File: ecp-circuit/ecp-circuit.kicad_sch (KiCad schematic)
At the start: 11 parts, among them K1 SINGLE CH RELAY, K2 DUAL CHANNEL RELAY, SW1 ON, SW2 OFF, T1 STEP DOWN

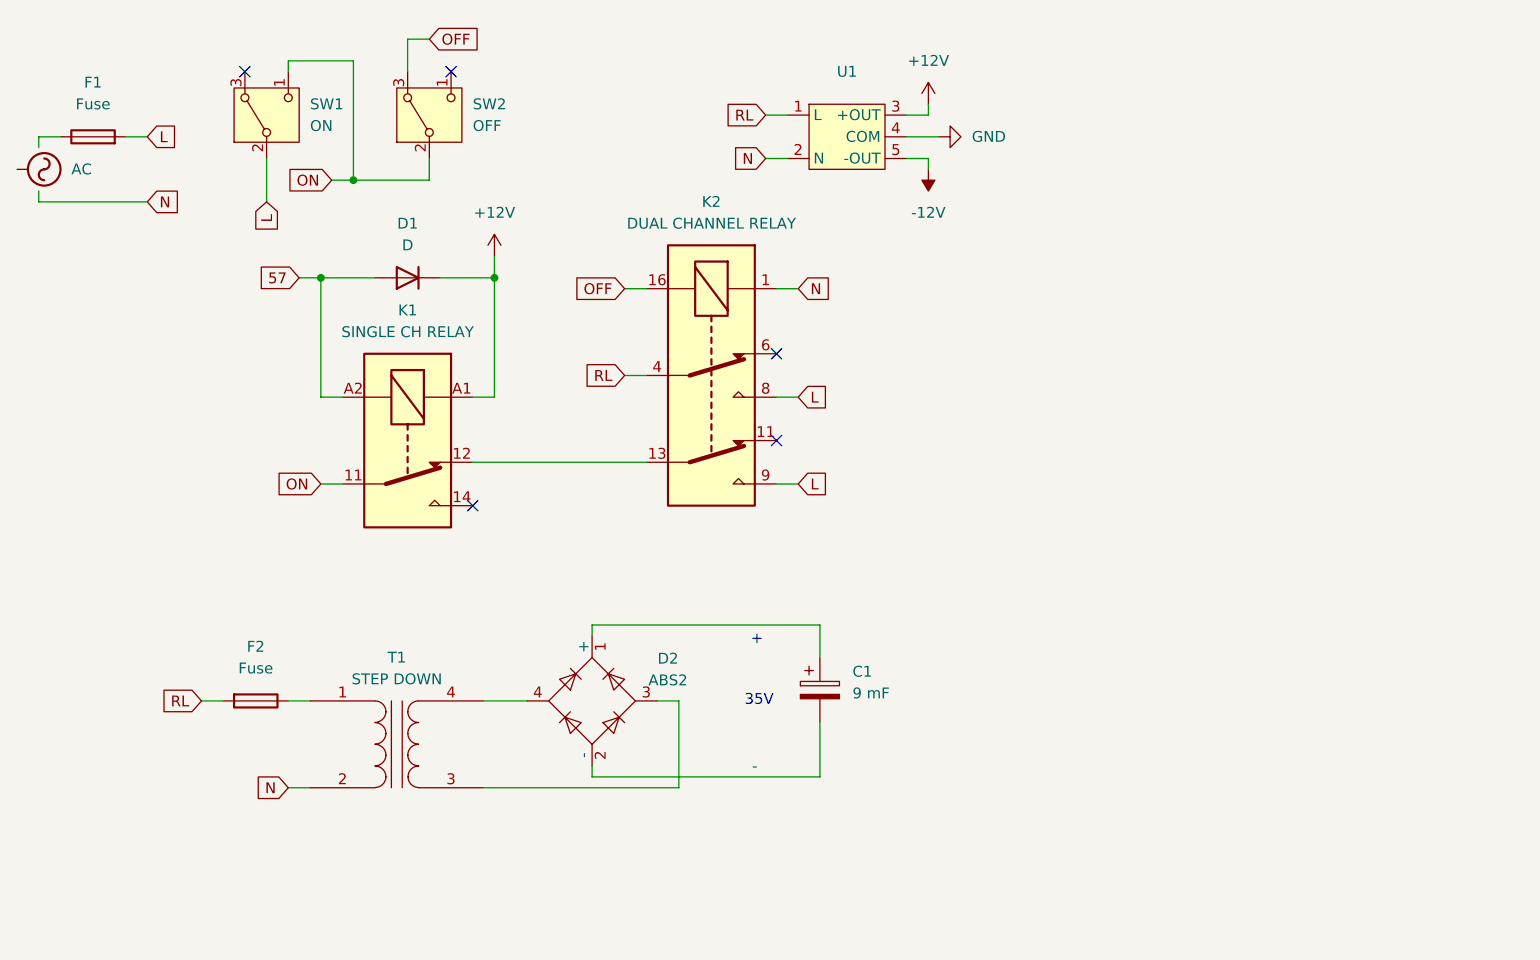
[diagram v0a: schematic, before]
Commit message: Update
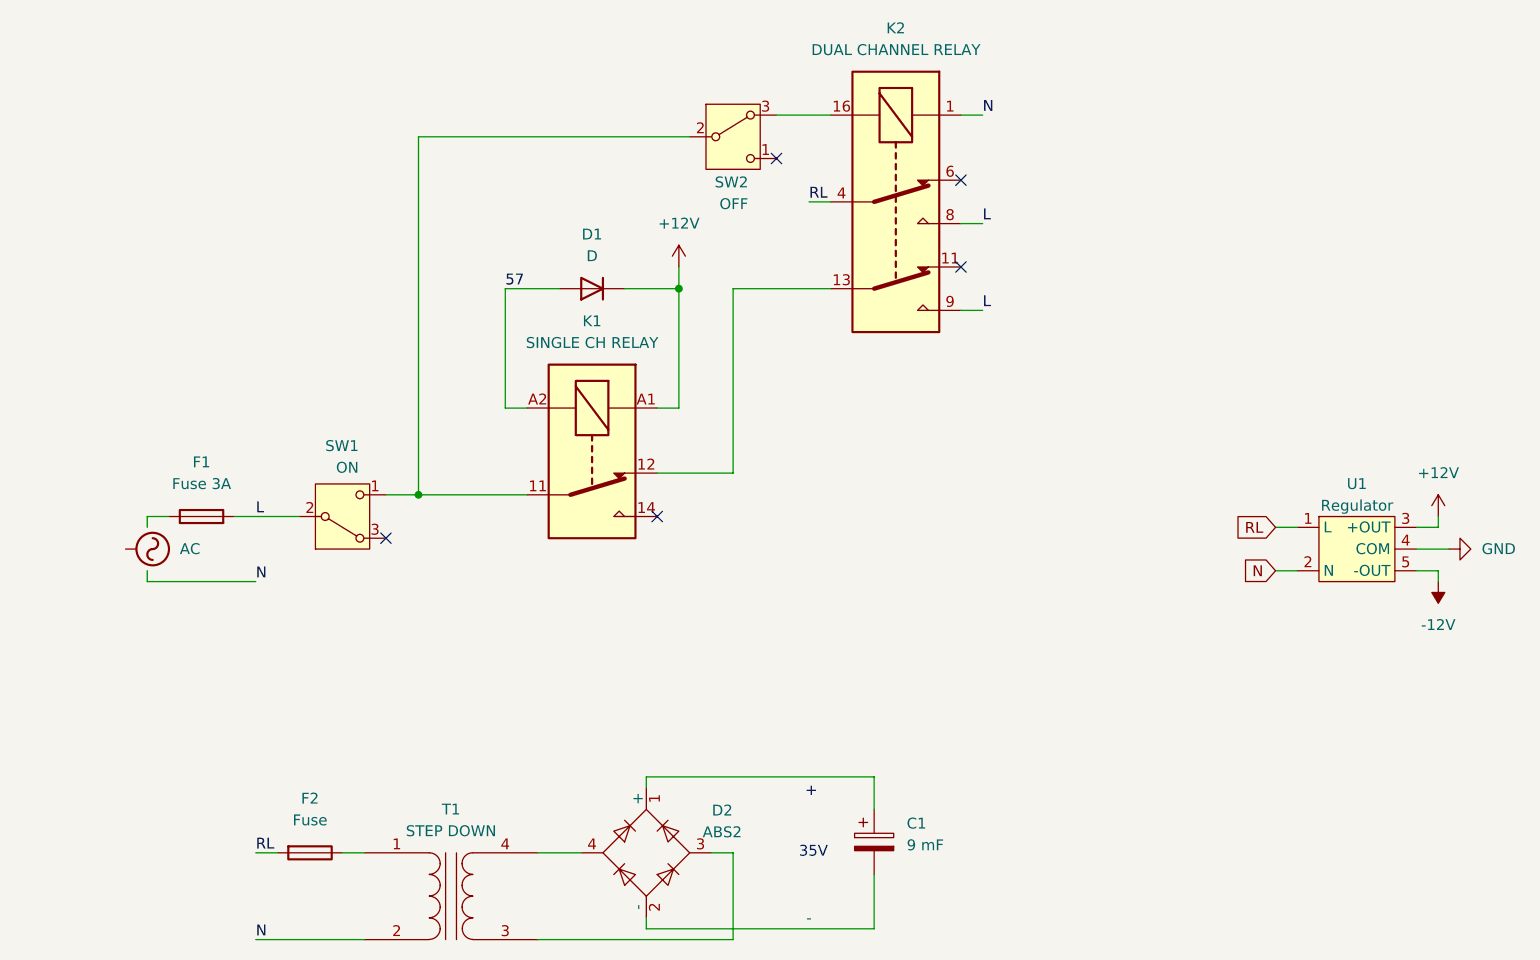
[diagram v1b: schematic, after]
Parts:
- F1: value Fuse -> Fuse 3A
- U1: value ~ -> Regulator
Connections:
- net OFF: no longer names the net of K2.16, SW2.3 (A)
- net ON: no longer names the net of K1.11, SW1.1 (C), SW2.2 (B)
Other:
- moved on the sheet: C1, D1, D2, F1, F2, K1, K2, SW1, SW2, T1, U1
